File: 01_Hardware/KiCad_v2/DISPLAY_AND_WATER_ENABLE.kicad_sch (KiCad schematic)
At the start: 30 parts, among them J700 JST_B4B, J701 JST_B4B, Q700 BSS314PEH6327, Q701 BSS314PEH6327, Q702 IRLML2402TRPBF, Q703 IRLML2402TRPBF

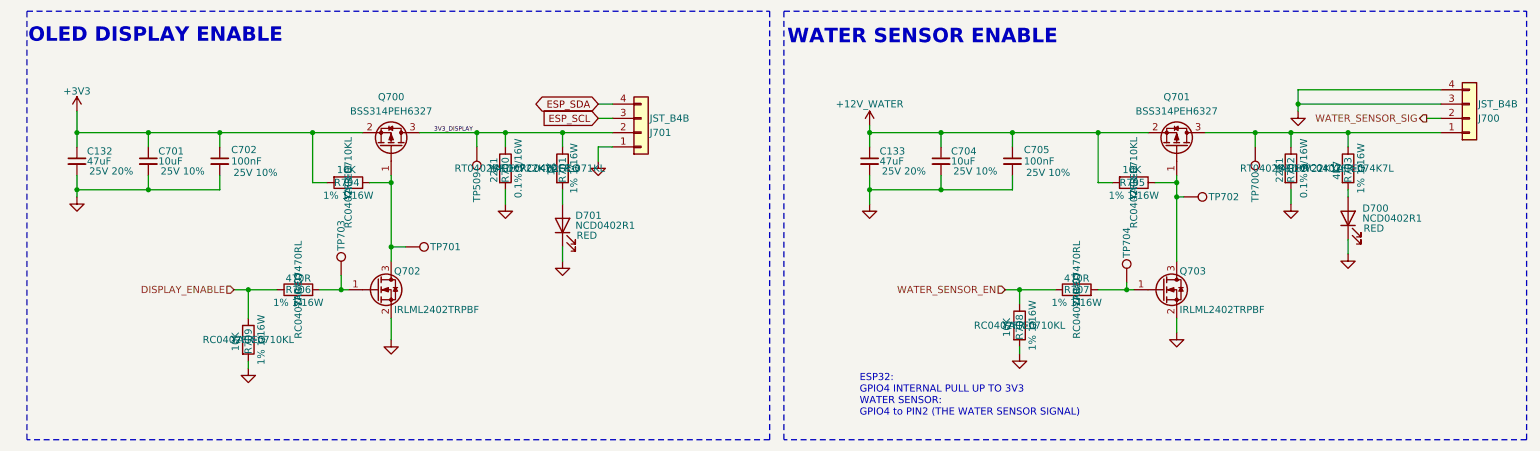
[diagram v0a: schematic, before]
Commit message: USB-C and Serial PCB routing done
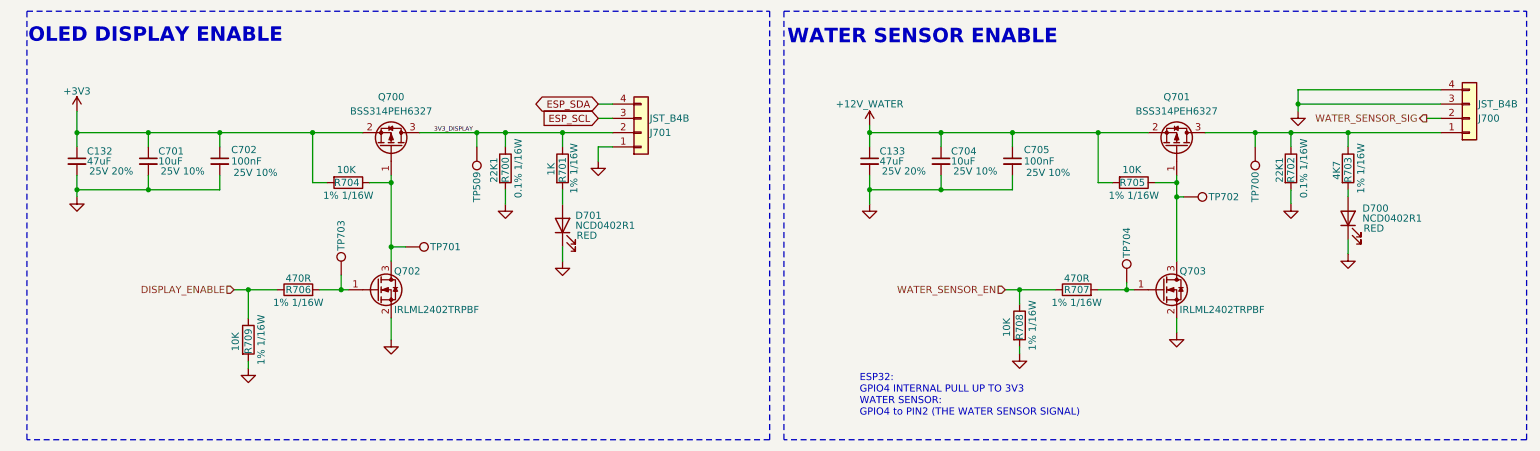
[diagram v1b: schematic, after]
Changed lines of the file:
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@@
 					(size 1.27 1.27)
 				)
+				(hide yes)
 			)
 		)
@@
 					(size 1.27 1.27)
 				)
+				(hide yes)
 			)
 		)
@@
 					(size 1.27 1.27)
 				)
+				(hide yes)
 			)
 		)
@@
 					(size 1.27 1.27)
 				)
+				(hide yes)
 			)
 		)
@@
 					(size 1.27 1.27)
 				)
+				(hide yes)
 			)
 		)
@@
 					(size 1.27 1.27)
 				)
+				(hide yes)
 			)
 		)
@@
 					(size 1.27 1.27)
 				)
+				(hide yes)
 			)
 		)
@@
 					(size 1.27 1.27)
 				)
+				(hide yes)
 			)
 		)
@@
 					(size 1.27 1.27)
 				)
+				(hide yes)
 			)
 		)
@@
 					(size 1.27 1.27)
 				)
+				(hide yes)
 			)
 		)
@@
 					(size 1.27 1.27)
 				)
+				(hide yes)
 			)
 		)
@@
 					(size 1.27 1.27)
 				)
+				(hide yes)
 			)
 		)
@@
 					(size 1.27 1.27)
 				)
+				(hide yes)
 			)
 		)
@@
 					(size 1.27 1.27)
 				)
+				(hide yes)
 			)
 		)
@@
 					(size 1.27 1.27)
 				)
+				(hide yes)
 			)
 		)
@@
 					(size 1.27 1.27)
 				)
+				(hide yes)
 			)
 		)
@@
 					(size 1.27 1.27)
 				)
+				(hide yes)
 			)
 		)
@@
 					(size 1.27 1.27)
 				)
+				(hide yes)
 			)
 		)
@@
 					(size 1.27 1.27)
 				)
+				(hide yes)
 			)
 		)
@@
 					(size 1.27 1.27)
 				)
+				(hide yes)
 			)
 		)
@@
 					(size 1.27 1.27)
 				)
+				(hide yes)
 			)
 		)
@@
 					(size 1.27 1.27)
 				)
+				(hide yes)
 			)
 		)
@@
 					(size 1.27 1.27)
 				)
+				(hide yes)
 			)
 		)
@@
 					(size 1.27 1.27)
 				)
+				(hide yes)
 			)
 		)
@@
 					(size 1.27 1.27)
 				)
+				(hide yes)
 			)
 		)
@@
 					(size 1.27 1.27)
 				)
+				(hide yes)
 			)
 		)
@@
 					(size 1.27 1.27)
 				)
+				(hide yes)
 			)
 		)
@@
 					(size 1.27 1.27)
 				)
+				(hide yes)
 			)
 		)
@@
 					(size 1.27 1.27)
 				)
+				(hide yes)
 			)
 		)
@@
 					(size 1.27 1.27)
 				)
+				(hide yes)
 			)
 		)
@@
 					(size 1.27 1.27)
 				)
+				(hide yes)
 			)
 		)
@@
 					(size 1.27 1.27)
 				)
+				(hide yes)
 			)
 		)
@@
 					(size 1.27 1.27)
 				)
+				(hide yes)
 			)
 		)
@@
 					(size 1.27 1.27)
 				)
+				(hide yes)
 			)
 		)
@@
 					(size 1.27 1.27)
 				)
+				(hide yes)
 			)
 		)
@@
 					(size 1.27 1.27)
 				)
+				(hide yes)
 			)
 		)
@@
 					(size 1.27 1.27)
 				)
+				(hide yes)
 			)
 		)
@@
 					(size 1.27 1.27)
 				)
+				(hide yes)
 			)
 		)
@@
 					(size 1.27 1.27)
 				)
+				(hide yes)
 			)
 		)
@@
 					(size 1.27 1.27)
 				)
-			)
-		)
+				(hide yes)
+			)
+		)
